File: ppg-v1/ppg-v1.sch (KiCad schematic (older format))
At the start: 56 parts, among them J1 USB_microB_2040002-1, J2 Conn_01x04_Male, SW1 SW_Push, SW2 SW_Push, SW3 PCM12, U1 STM32F411CEUx, U2 MCP73831T-2ACI/OT, U3 Opamp_Dual_Generic, U4 Opamp_Dual_Generic, U5 TPS2113APW, U6 MCP1702T-3302E/CB, U7 BM71BLES1FC2, Y1 12MHz, Y2 32K768

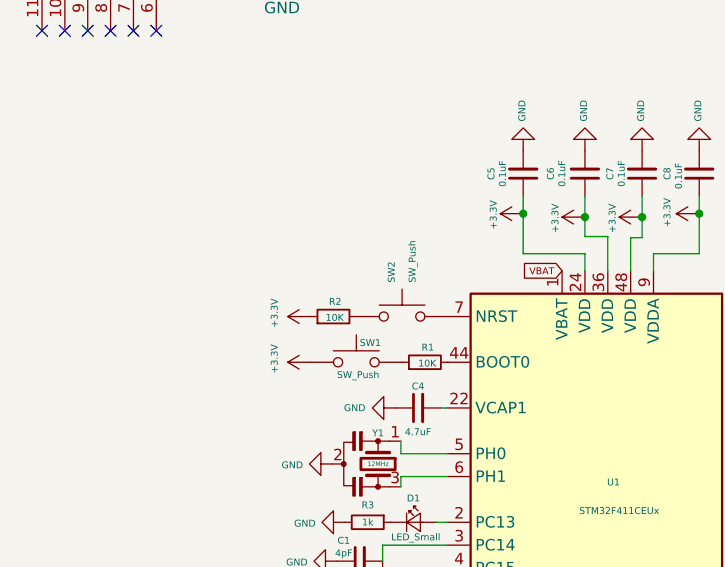
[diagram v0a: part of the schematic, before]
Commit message: fix buttons
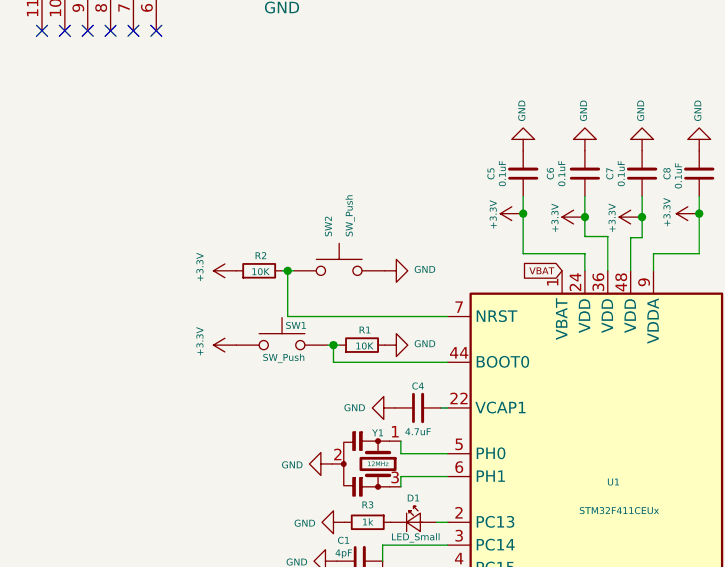
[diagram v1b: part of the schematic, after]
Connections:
- wire segments 154 -> 162
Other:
- moved on the sheet: R1, R2, SW1, SW2
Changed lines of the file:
@@
 EESchema Schematic File Version 4
 LIBS:ppg-v1-cache
-EELAYER 26 0
+EELAYER 29 0
 EELAYER END
 $Descr A4 11693 8268
@@
 L Device:R_Small R2
 U 1 1 5CAD0F8E
-P 2000 3275
-F 0 "R2" V 2065 3240 30  0000 L CNN
-F 1 "10K" V 1995 3230 30  0000 L CNN
-F 2 "Resistor_SMD:R_0603_1608Metric" H 2000 3275 30  0001 C CNN
-F 3 "~" H 2000 3275 30  0001 C CNN
-	1    2000 3275
+P 1675 3075
+F 0 "R2" V 1740 3040 30  0000 L CNN
+F 1 "10K" V 1670 3030 30  0000 L CNN
+F 2 "Resistor_SMD:R_0603_1608Metric" H 1675 3075 30  0001 C CNN
+F 3 "~" H 1675 3075 30  0001 C CNN
+	1    1675 3075
 	0    -1   -1   0
 $EndComp
@@
 L Device:R_Small R1
 U 1 1 5CAD3717
-P 2400 3475
-F 0 "R1" V 2465 3435 30  0000 L CNN
-F 1 "10K" V 2395 3425 30  0000 L CNN
-F 2 "Resistor_SMD:R_0603_1608Metric" H 2400 3475 30  0001 C CNN
-F 3 "~" H 2400 3475 30  0001 C CNN
-	1    2400 3475
+P 2125 3400
+F 0 "R1" V 2190 3360 30  0000 L CNN
+F 1 "10K" V 2120 3350 30  0000 L CNN
+F 2 "Resistor_SMD:R_0603_1608Metric" H 2125 3400 30  0001 C CNN
+F 3 "~" H 2125 3400 30  0001 C CNN
+	1    2125 3400
 	0    -1   -1   0
 $EndComp
@@
 L Switch:SW_Push SW1
 U 1 1 5CAD40DA
-P 2100 3475
-F 0 "SW1" H 2115 3560 30  0000 L CNN
-F 1 "SW_Push" H 2015 3420 30  0000 L CNN
-F 2 "Button_Switch_SMD:SW_SPST_B3U-1000P" H 2100 3675 30  0001 C CNN
-F 3 "~" H 2100 3675 30  0001 C CNN
-	1    2100 3475
+P 1775 3400
+F 0 "SW1" H 1790 3485 30  0000 L CNN
+F 1 "SW_Push" H 1690 3345 30  0000 L CNN
+F 2 "Button_Switch_SMD:SW_SPST_B3U-1000P" H 1775 3600 30  0001 C CNN
+F 3 "~" H 1775 3600 30  0001 C CNN
+	1    1775 3400
 	1    0    0    -1
 $EndComp
@@
 L Switch:SW_Push SW2
 U 1 1 5CAE2F2D
-P 2300 3275
-F 0 "SW2" V 2254 3423 30  0000 L CNN
-F 1 "SW_Push" V 2345 3423 30  0000 L CNN
-F 2 "Button_Switch_SMD:SW_SPST_B3U-1000P" H 2300 3475 30  0001 C CNN
-F 3 "~" H 2300 3475 30  0001 C CNN
-	1    2300 3275
+P 2025 3075
+F 0 "SW2" V 1979 3223 30  0000 L CNN
+F 1 "SW_Push" V 2070 3223 30  0000 L CNN
+F 2 "Button_Switch_SMD:SW_SPST_B3U-1000P" H 2025 3275 30  0001 C CNN
+F 3 "~" H 2025 3275 30  0001 C CNN
+	1    2025 3075
 	1    0    0    -1
 $EndComp
@@
 L power:+3.3V #PWR06
 U 1 1 5CAC3018
-P 1900 3275
-F 0 "#PWR06" H 1900 3125 30  0001 C CNN
-F 1 "+3.3V" H 1915 3433 30  0000 C CNN
-F 2 "" H 1900 3275 30  0001 C CNN
-F 3 "" H 1900 3275 30  0001 C CNN
-	1    1900 3275
+P 1575 3075
+F 0 "#PWR06" H 1575 2925 30  0001 C CNN
+F 1 "+3.3V" H 1590 3233 30  0000 C CNN
+F 2 "" H 1575 3075 30  0001 C CNN
+F 3 "" H 1575 3075 30  0001 C CNN
+	1    1575 3075
 	0    -1   -1   0
 $EndComp
@@
 L power:+3.3V #PWR01
 U 1 1 5CAC33BF
-P 1900 3475
-F 0 "#PWR01" H 1900 3325 30  0001 C CNN
-F 1 "+3.3V" H 1915 3633 30  0000 C CNN
-F 2 "" H 1900 3475 30  0001 C CNN
-F 3 "" H 1900 3475 30  0001 C CNN
-	1    1900 3475
+P 1575 3400
+F 0 "#PWR01" H 1575 3250 30  0001 C CNN
+F 1 "+3.3V" H 1590 3558 30  0000 C CNN
+F 2 "" H 1575 3400 30  0001 C CNN
+F 3 "" H 1575 3400 30  0001 C CNN
+	1    1575 3400
 	0    -1   -1   0
 $EndComp
@@
 Wire Wire Line
 	1810 6380 1810 6375
+$Comp
+L power:GND #PWR?
+U 1 1 5CB9CAA7
+P 2225 3075
+F 0 "#PWR?" H 2225 2825 30  0001 C CNN
+F 1 "GND" V 2230 2947 30  0000 R CNN
+F 2 "" H 2225 3075 30  0001 C CNN
+F 3 "" H 2225 3075 30  0001 C CNN
+	1    2225 3075
+	0    -1   -1   0
+$EndComp
+$Comp
+L power:GND #PWR?
+U 1 1 5CB9CFB0
+P 2225 3400
+F 0 "#PWR?" H 2225 3150 30  0001 C CNN
+F 1 "GND" V 2230 3272 30  0000 R CNN
+F 2 "" H 2225 3400 30  0001 C CNN
+F 3 "" H 2225 3400 30  0001 C CNN
+	1    2225 3400
+	0    -1   -1   0
+$EndComp
+Wire Wire Line
+	1775 3075 1800 3075
+Wire Wire Line
+	1800 3075 1800 3275
+Wire Wire Line
+	1800 3275 2500 3275
+Connection ~ 1800 3075
+Wire Wire Line
+	1800 3075 1825 3075
+Wire Wire Line
+	1975 3400 2000 3400
+Wire Wire Line
+	2000 3400 2000 3475
+Wire Wire Line
+	2000 3475 2500 3475
+Connection ~ 2000 3400
+Wire Wire Line
+	2000 3400 2025 3400
 $EndSCHEMATC
